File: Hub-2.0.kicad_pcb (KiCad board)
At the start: 2 copper layers, 120 x 100 mm, 17 parts, among them CN4 DT15-12PA, CN5 DT15-12PA, CN6 DT15-12PA, J10-PCB1 5569-16A2, J2-PCB1 5569-20A2, J3-PCB1 5569-06A2, J4-PCB1 5569-08A2, J5-PCB1 5569-18A2

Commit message: Autosave
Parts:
- moved J4-PCB1 119.6 mm to (217.7, 68.7)
- moved H1 119.6 mm to (211.9, -2.00)
- moved H2 119.6 mm to (211.9, 91.0)
- moved J2-PCB1 119.6 mm to (219.0, 3.77)
- moved J5-PCB1 119.6 mm to (217.7, 49.4)
- moved H4 119.6 mm to (304.9, -2.00)
- moved J10-PCB1 119.6 mm to (268.7, 3.77)
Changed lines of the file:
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@@
 	(footprint "MountingHole:MountingHole_3.2mm_M3_Pad_Via"
 		(layer "F.Cu")
-		(at 105.7 53.025)
+		(at 211.9 -2)
 		(descr "Mounting Hole 3.2mm, M3")
 		(tags "mounting hole 3.2mm m3")
@@
 	(footprint "MountingHole:MountingHole_3.2mm_M3_Pad_Via"
 		(layer "F.Cu")
-		(at 105.7 146.025)
+		(at 211.9 91)
 		(descr "Mounting Hole 3.2mm, M3")
 		(tags "mounting hole 3.2mm m3")
@@
 	(footprint "MountingHole:MountingHole_3.2mm_M3_Pad_Via"
 		(layer "F.Cu")
-		(at 198.7 53.025)
+		(at 304.9 -2)
 		(descr "Mounting Hole 3.2mm, M3")
 		(tags "mounting hole 3.2mm m3")
@@
 	(footprint "Connector_Molex:Molex_Mini-Fit_Jr_5569-16A2_2x08_P4.20mm_Horizontal"
 		(layer "F.Cu")
-		(at 162.5 58.8)
+		(at 268.7 3.775)
 		(descr "Molex Mini-Fit Jr. Power Connectors, old mpn/engineering number: 5569-16A2, example for new mpn: 39-30-0160, 8 Pins per row, Mounting: Snap-in Plastic Peg PCB Lock (http://www.molex.com/pdm_docs/sd/039300020_sd.pdf)")
 		(tags "connector Molex Mini-Fit_Jr horizontalplastic_peg")
@@
 	(footprint "Connector_Molex:Molex_Mini-Fit_Jr_5569-08A2_2x04_P4.20mm_Horizontal"
 		(layer "F.Cu")
-		(at 111.475 123.725 90)
+		(at 217.675 68.7 90)
 		(descr "Molex Mini-Fit Jr. Power Connectors, old mpn/engineering number: 5569-08A2, example for new mpn: 39-30-0080, 4 Pins per row, Mounting: Snap-in Plastic Peg PCB Lock (http://www.molex.com/pdm_docs/sd/039300020_sd.pdf)")
 		(tags "connector Molex Mini-Fit_Jr horizontalplastic_peg")
@@
 	(footprint "Connector_Molex:Molex_Mini-Fit_Jr_5569-20A2_2x10_P4.20mm_Horizontal"
 		(layer "F.Cu")
-		(at 112.8 58.8)
+		(at 219 3.775)
 		(descr "Molex Mini-Fit Jr. Power Connectors, old mpn/engineering number: 5569-20A2, example for new mpn: 39-30-0200, 10 Pins per row, Mounting: Snap-in Plastic Peg PCB Lock (http://www.molex.com/pdm_docs/sd/039300020_sd.pdf)")
 		(tags "connector Molex Mini-Fit_Jr horizontalplastic_peg")
@@
 	(footprint "Connector_Molex:Molex_Mini-Fit_Jr_5569-18A2_2x09_P4.20mm_Horizontal"
 		(layer "F.Cu")
-		(at 111.45 104.375 90)
+		(at 217.65 49.35 90)
 		(descr "Molex Mini-Fit Jr. Power Connectors, old mpn/engineering number: 5569-18A2, example for new mpn: 39-30-0180, 9 Pins per row, Mounting: Snap-in Plastic Peg PCB Lock (http://www.molex.com/pdm_docs/sd/039300020_sd.pdf)")
 		(tags "connector Molex Mini-Fit_Jr horizontalplastic_peg")
@@
 	)
 	(gr_rect
-		(start 101.81 49.07)
-		(end 221.81 149.07)
+		(start 208.4 -5.4)
+		(end 328.4 94.6)
 		(stroke
 			(width 0.2)
@@
 	)
 	(gr_line
-		(start 102.2 53.025)
-		(end 102.2 146.025)
+		(start 208.4 -2)
+		(end 208.4 91)
 		(stroke
 			(width 0.1)
@@
 	)
 	(gr_arc
-		(start 102.2 53.025)
-		(mid 103.225126 50.550126)
-		(end 105.7 49.525)
+		(start 208.4 -2)
+		(mid 209.425126 -4.474874)
+		(end 211.9 -5.5)
 		(stroke
 			(width 0.1)
@@
 	)
 	(gr_arc
-		(start 105.7 149.525)
-		(mid 103.225126 148.499874)
-		(end 102.2 146.025)
+		(start 211.9 94.5)
+		(mid 209.425126 93.474874)
+		(end 208.4 91)
 		(stroke
 			(width 0.1)
@@
 	)
 	(gr_line
-		(start 105.7 149.525)
-		(end 198.7 149.525)
+		(start 211.9 94.5)
+		(end 304.9 94.5)
 		(stroke
 			(width 0.1)
@@
 	)
 	(gr_line
-		(start 198.7 49.525)
-		(end 105.7 49.525)
+		(start 304.9 -5.5)
+		(end 211.9 -5.5)
 		(stroke
 			(width 0.1)
@@
 	)
 	(gr_arc
-		(start 198.7 49.525)
-		(mid 201.174874 50.550126)
-		(end 202.2 53.025)
+		(start 304.9 -5.5)
+		(mid 307.374874 -4.474874)
+		(end 308.4 -2)
 		(stroke
 			(width 0.1)
@@
 	)
 	(gr_arc
-		(start 202.2 146.025)
-		(mid 201.174874 148.499874)
-		(end 198.7 149.525)
+		(start 308.4 91)
+		(mid 307.374874 93.474874)
+		(end 304.9 94.5)
 		(stroke
 			(width 0.1)
@@
 	)
 	(gr_line
-		(start 202.2 146.025)
-		(end 202.2 53.025)
+		(start 308.4 91)
+		(end 308.4 -2)
 		(stroke
 			(width 0.1)
@@
 	)
 	(segment
-		(start 152.12 78.54)
-		(end 152.08 78.5)
+		(start 258.32 23.515)
+		(end 258.28 23.475)
 		(width 0.2)
 		(layer "F.Cu")

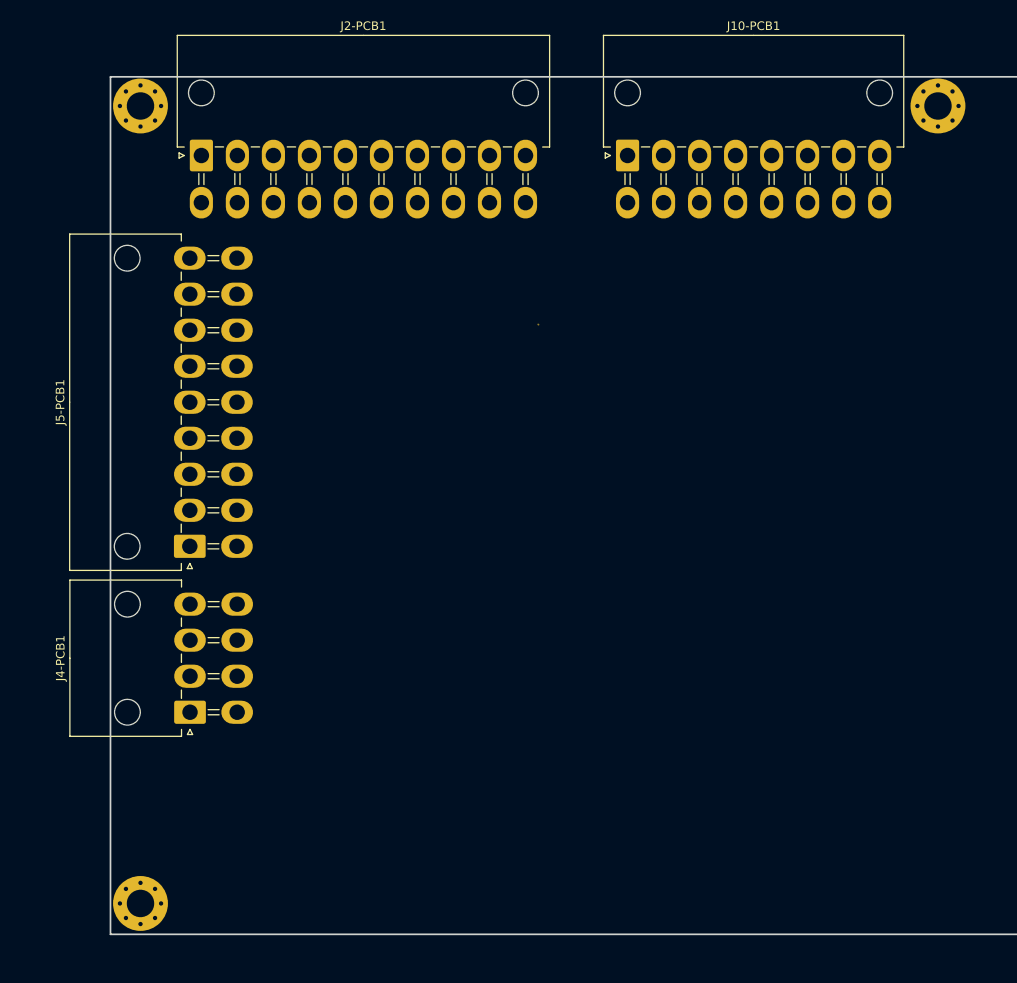
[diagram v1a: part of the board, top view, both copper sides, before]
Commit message: Autosave
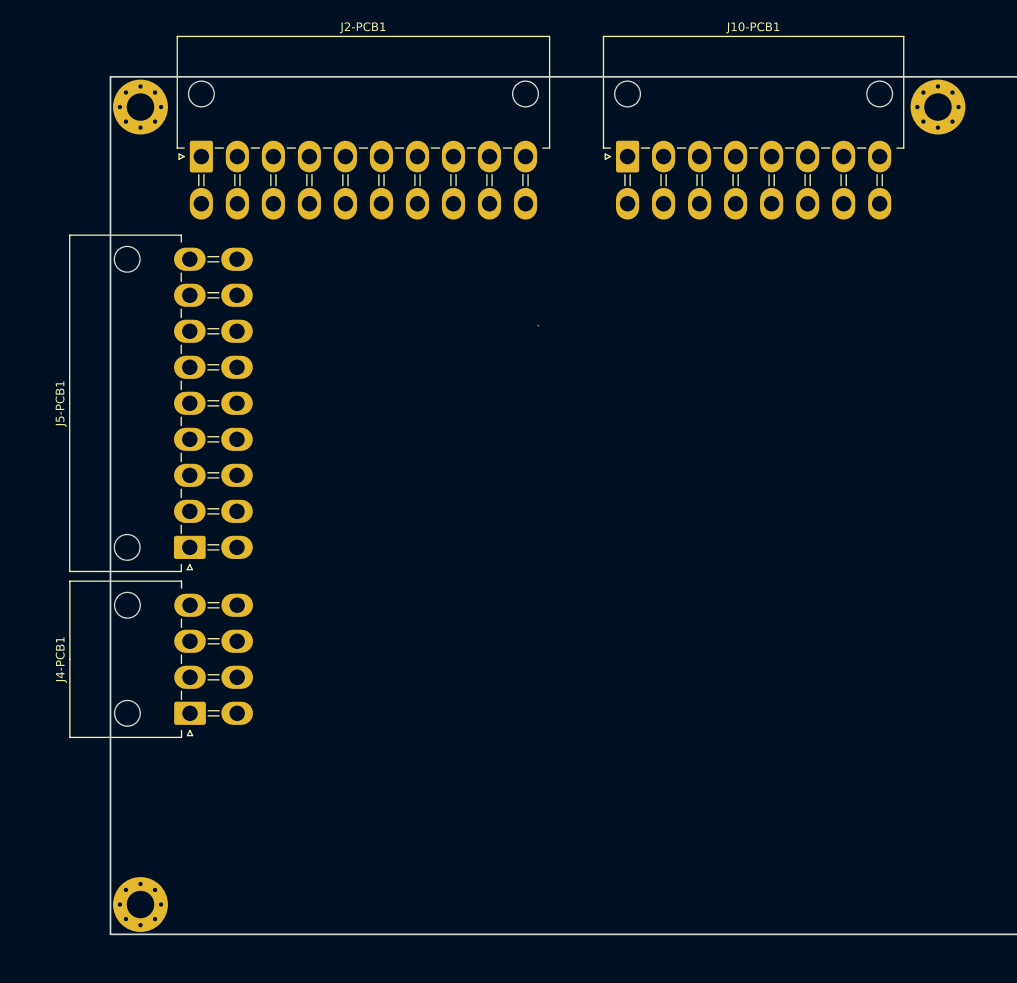
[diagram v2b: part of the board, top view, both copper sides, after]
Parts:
- moved H1 0.12 mm to (211.9, -1.88)
- moved H2 0.12 mm to (211.9, 91.1)
- moved H4 0.12 mm to (304.9, -1.88)
- moved J10-PCB1 0.12 mm to (268.7, 3.90)
- moved J2-PCB1 0.12 mm to (219.0, 3.90)
- moved J4-PCB1 0.12 mm to (217.7, 68.8)
- moved J5-PCB1 0.12 mm to (217.7, 49.5)
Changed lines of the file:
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@@
 	(footprint "MountingHole:MountingHole_3.2mm_M3_Pad_Via"
 		(layer "F.Cu")
-		(at 211.9 -2)
+		(at 211.9 -1.875)
 		(descr "Mounting Hole 3.2mm, M3")
 		(tags "mounting hole 3.2mm m3")
@@
 	(footprint "MountingHole:MountingHole_3.2mm_M3_Pad_Via"
 		(layer "F.Cu")
-		(at 211.9 91)
+		(at 211.9 91.125)
 		(descr "Mounting Hole 3.2mm, M3")
 		(tags "mounting hole 3.2mm m3")
@@
 	(footprint "MountingHole:MountingHole_3.2mm_M3_Pad_Via"
 		(layer "F.Cu")
-		(at 304.9 -2)
+		(at 304.9 -1.875)
 		(descr "Mounting Hole 3.2mm, M3")
 		(tags "mounting hole 3.2mm m3")
@@
 	(footprint "Connector_Molex:Molex_Mini-Fit_Jr_5569-16A2_2x08_P4.20mm_Horizontal"
 		(layer "F.Cu")
-		(at 268.7 3.775)
+		(at 268.7 3.9)
 		(descr "Molex Mini-Fit Jr. Power Connectors, old mpn/engineering number: 5569-16A2, example for new mpn: 39-30-0160, 8 Pins per row, Mounting: Snap-in Plastic Peg PCB Lock (http://www.molex.com/pdm_docs/sd/039300020_sd.pdf)")
 		(tags "connector Molex Mini-Fit_Jr horizontalplastic_peg")
@@
 	(footprint "Connector_Molex:Molex_Mini-Fit_Jr_5569-08A2_2x04_P4.20mm_Horizontal"
 		(layer "F.Cu")
-		(at 217.675 68.7 90)
+		(at 217.675 68.825 90)
 		(descr "Molex Mini-Fit Jr. Power Connectors, old mpn/engineering number: 5569-08A2, example for new mpn: 39-30-0080, 4 Pins per row, Mounting: Snap-in Plastic Peg PCB Lock (http://www.molex.com/pdm_docs/sd/039300020_sd.pdf)")
 		(tags "connector Molex Mini-Fit_Jr horizontalplastic_peg")
@@
 	(footprint "Connector_Molex:Molex_Mini-Fit_Jr_5569-20A2_2x10_P4.20mm_Horizontal"
 		(layer "F.Cu")
-		(at 219 3.775)
+		(at 219 3.9)
 		(descr "Molex Mini-Fit Jr. Power Connectors, old mpn/engineering number: 5569-20A2, example for new mpn: 39-30-0200, 10 Pins per row, Mounting: Snap-in Plastic Peg PCB Lock (http://www.molex.com/pdm_docs/sd/039300020_sd.pdf)")
 		(tags "connector Molex Mini-Fit_Jr horizontalplastic_peg")
@@
 	(footprint "Connector_Molex:Molex_Mini-Fit_Jr_5569-18A2_2x09_P4.20mm_Horizontal"
 		(layer "F.Cu")
-		(at 217.65 49.35 90)
+		(at 217.65 49.475 90)
 		(descr "Molex Mini-Fit Jr. Power Connectors, old mpn/engineering number: 5569-18A2, example for new mpn: 39-30-0180, 9 Pins per row, Mounting: Snap-in Plastic Peg PCB Lock (http://www.molex.com/pdm_docs/sd/039300020_sd.pdf)")
 		(tags "connector Molex Mini-Fit_Jr horizontalplastic_peg")
@@
 	)
 	(gr_line
-		(start 208.4 -2)
-		(end 208.4 91)
+		(start 208.4 -1.875)
+		(end 208.4 91.125)
 		(stroke
 			(width 0.1)
@@
 	)
 	(gr_arc
-		(start 208.4 -2)
-		(mid 209.425126 -4.474874)
-		(end 211.9 -5.5)
+		(start 208.4 -1.875)
+		(mid 209.425126 -4.349874)
+		(end 211.9 -5.375)
 		(stroke
 			(width 0.1)
@@
 	)
 	(gr_arc
-		(start 211.9 94.5)
-		(mid 209.425126 93.474874)
-		(end 208.4 91)
+		(start 211.9 94.625)
+		(mid 209.425126 93.599874)
+		(end 208.4 91.125)
 		(stroke
 			(width 0.1)
@@
 	)
 	(gr_line
-		(start 211.9 94.5)
-		(end 304.9 94.5)
+		(start 211.9 94.625)
+		(end 304.9 94.625)
 		(stroke
 			(width 0.1)
@@
 	)
 	(gr_line
-		(start 304.9 -5.5)
-		(end 211.9 -5.5)
+		(start 304.9 -5.375)
+		(end 211.9 -5.375)
 		(stroke
 			(width 0.1)
@@
 	)
 	(gr_arc
-		(start 304.9 -5.5)
-		(mid 307.374874 -4.474874)
-		(end 308.4 -2)
+		(start 304.9 -5.375)
+		(mid 307.374874 -4.349874)
+		(end 308.4 -1.875)
 		(stroke
 			(width 0.1)
@@
 	)
 	(gr_arc
-		(start 308.4 91)
-		(mid 307.374874 93.474874)
-		(end 304.9 94.5)
+		(start 308.4 91.125)
+		(mid 307.374874 93.599874)
+		(end 304.9 94.625)
 		(stroke
 			(width 0.1)
@@
 	)
 	(gr_line
-		(start 308.4 91)
-		(end 308.4 -2)
+		(start 308.4 91.125)
+		(end 308.4 -1.875)
 		(stroke
 			(width 0.1)
@@
 	)
 	(segment
-		(start 258.32 23.515)
-		(end 258.28 23.475)
+		(start 258.32 23.64)
+		(end 258.28 23.6)
 		(width 0.2)
 		(layer "F.Cu")

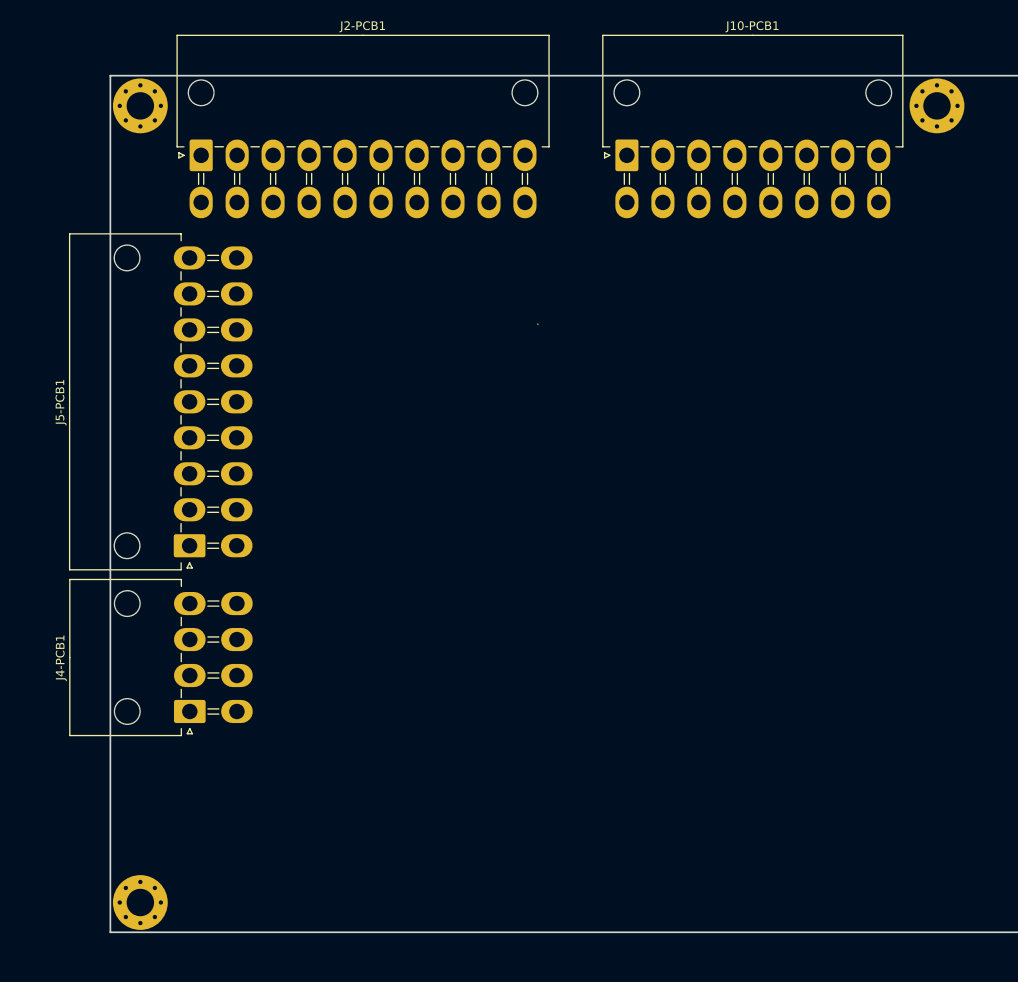
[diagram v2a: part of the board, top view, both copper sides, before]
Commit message: PCB Save
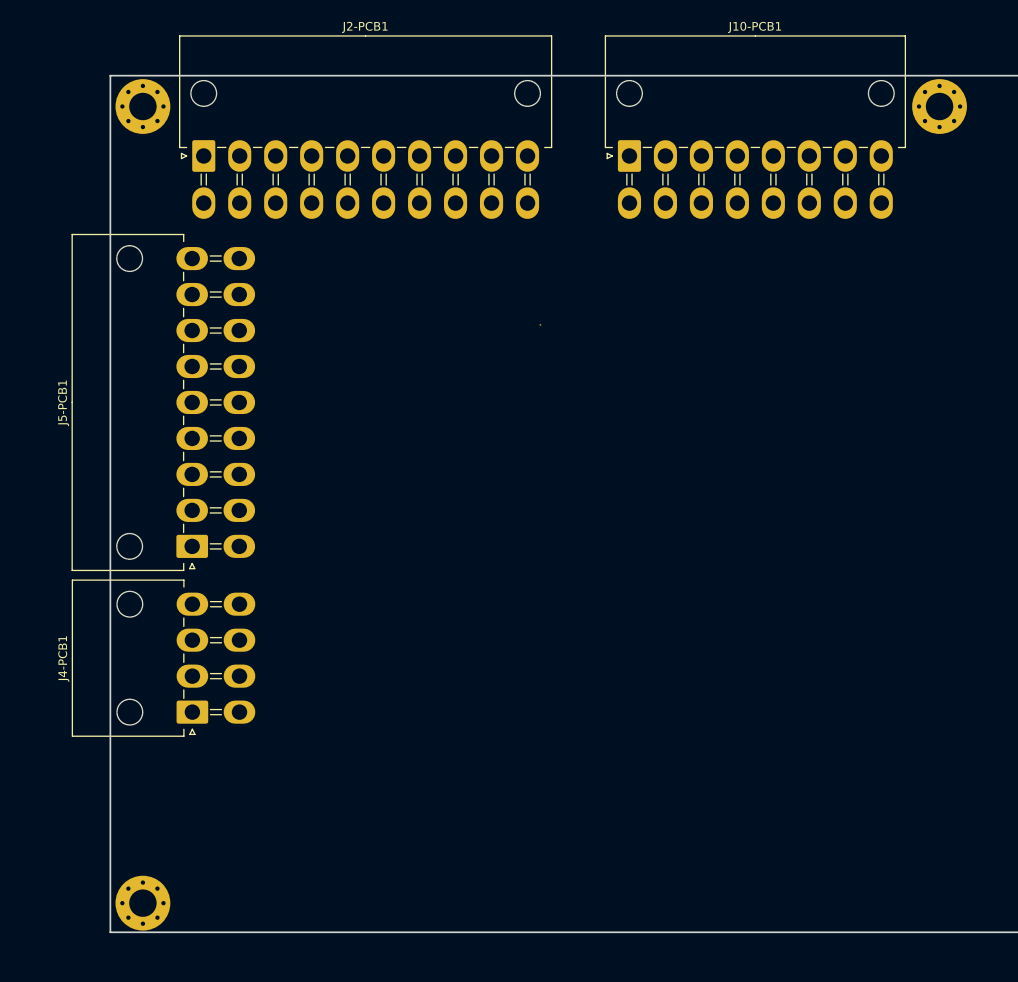
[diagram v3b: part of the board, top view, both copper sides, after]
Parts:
- moved J10-PCB1 0.31 mm to (269.0, 3.98)
- moved J2-PCB1 0.31 mm to (219.3, 3.98)
- moved H4 0.31 mm to (305.2, -1.80)
- moved H2 0.31 mm to (212.2, 91.2)
- moved J4-PCB1 0.31 mm to (218.0, 68.9)
- moved H1 0.31 mm to (212.2, -1.80)
- moved J5-PCB1 0.31 mm to (217.9, 49.5)
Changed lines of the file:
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@@
 	(footprint "MountingHole:MountingHole_3.2mm_M3_Pad_Via"
 		(layer "F.Cu")
-		(at 211.9 -1.875)
+		(at 212.2 -1.8)
 		(descr "Mounting Hole 3.2mm, M3")
 		(tags "mounting hole 3.2mm m3")
@@
 	(footprint "MountingHole:MountingHole_3.2mm_M3_Pad_Via"
 		(layer "F.Cu")
-		(at 211.9 91.125)
+		(at 212.2 91.2)
 		(descr "Mounting Hole 3.2mm, M3")
 		(tags "mounting hole 3.2mm m3")
@@
 	(footprint "MountingHole:MountingHole_3.2mm_M3_Pad_Via"
 		(layer "F.Cu")
-		(at 304.9 -1.875)
+		(at 305.2 -1.8)
 		(descr "Mounting Hole 3.2mm, M3")
 		(tags "mounting hole 3.2mm m3")
@@
 	(footprint "Connector_Molex:Molex_Mini-Fit_Jr_5569-16A2_2x08_P4.20mm_Horizontal"
 		(layer "F.Cu")
-		(at 268.7 3.9)
+		(at 269 3.975)
 		(descr "Molex Mini-Fit Jr. Power Connectors, old mpn/engineering number: 5569-16A2, example for new mpn: 39-30-0160, 8 Pins per row, Mounting: Snap-in Plastic Peg PCB Lock (http://www.molex.com/pdm_docs/sd/039300020_sd.pdf)")
 		(tags "connector Molex Mini-Fit_Jr horizontalplastic_peg")
@@
 	(footprint "Connector_Molex:Molex_Mini-Fit_Jr_5569-08A2_2x04_P4.20mm_Horizontal"
 		(layer "F.Cu")
-		(at 217.675 68.825 90)
+		(at 217.975 68.9 90)
 		(descr "Molex Mini-Fit Jr. Power Connectors, old mpn/engineering number: 5569-08A2, example for new mpn: 39-30-0080, 4 Pins per row, Mounting: Snap-in Plastic Peg PCB Lock (http://www.molex.com/pdm_docs/sd/039300020_sd.pdf)")
 		(tags "connector Molex Mini-Fit_Jr horizontalplastic_peg")
@@
 	(footprint "Connector_Molex:Molex_Mini-Fit_Jr_5569-20A2_2x10_P4.20mm_Horizontal"
 		(layer "F.Cu")
-		(at 219 3.9)
+		(at 219.3 3.975)
 		(descr "Molex Mini-Fit Jr. Power Connectors, old mpn/engineering number: 5569-20A2, example for new mpn: 39-30-0200, 10 Pins per row, Mounting: Snap-in Plastic Peg PCB Lock (http://www.molex.com/pdm_docs/sd/039300020_sd.pdf)")
 		(tags "connector Molex Mini-Fit_Jr horizontalplastic_peg")
@@
 	(footprint "Connector_Molex:Molex_Mini-Fit_Jr_5569-18A2_2x09_P4.20mm_Horizontal"
 		(layer "F.Cu")
-		(at 217.65 49.475 90)
+		(at 217.95 49.55 90)
 		(descr "Molex Mini-Fit Jr. Power Connectors, old mpn/engineering number: 5569-18A2, example for new mpn: 39-30-0180, 9 Pins per row, Mounting: Snap-in Plastic Peg PCB Lock (http://www.molex.com/pdm_docs/sd/039300020_sd.pdf)")
 		(tags "connector Molex Mini-Fit_Jr horizontalplastic_peg")
@@
 	)
 	(gr_line
-		(start 208.4 -1.875)
-		(end 208.4 91.125)
+		(start 208.7 -1.8)
+		(end 208.7 91.2)
 		(stroke
 			(width 0.1)
@@
 	)
 	(gr_arc
-		(start 208.4 -1.875)
-		(mid 209.425126 -4.349874)
-		(end 211.9 -5.375)
+		(start 208.7 -1.8)
+		(mid 209.725126 -4.274874)
+		(end 212.2 -5.3)
 		(stroke
 			(width 0.1)
@@
 	)
 	(gr_arc
-		(start 211.9 94.625)
-		(mid 209.425126 93.599874)
-		(end 208.4 91.125)
+		(start 212.2 94.7)
+		(mid 209.725126 93.674874)
+		(end 208.7 91.2)
 		(stroke
 			(width 0.1)
@@
 	)
 	(gr_line
-		(start 211.9 94.625)
-		(end 304.9 94.625)
+		(start 212.2 94.7)
+		(end 305.2 94.7)
 		(stroke
 			(width 0.1)
@@
 	)
 	(gr_line
-		(start 304.9 -5.375)
-		(end 211.9 -5.375)
+		(start 305.2 -5.3)
+		(end 212.2 -5.3)
 		(stroke
 			(width 0.1)
@@
 	)
 	(gr_arc
-		(start 304.9 -5.375)
-		(mid 307.374874 -4.349874)
-		(end 308.4 -1.875)
+		(start 305.2 -5.3)
+		(mid 307.674874 -4.274874)
+		(end 308.7 -1.8)
 		(stroke
 			(width 0.1)
@@
 	)
 	(gr_arc
-		(start 308.4 91.125)
-		(mid 307.374874 93.599874)
-		(end 304.9 94.625)
+		(start 308.7 91.2)
+		(mid 307.674874 93.674874)
+		(end 305.2 94.7)
 		(stroke
 			(width 0.1)
@@
 	)
 	(gr_line
-		(start 308.4 91.125)
-		(end 308.4 -1.875)
+		(start 308.7 91.2)
+		(end 308.7 -1.8)
 		(stroke
 			(width 0.1)
@@
 	)
 	(segment
-		(start 258.32 23.64)
-		(end 258.28 23.6)
+		(start 258.62 23.715)
+		(end 258.58 23.675)
 		(width 0.2)
 		(layer "F.Cu")
